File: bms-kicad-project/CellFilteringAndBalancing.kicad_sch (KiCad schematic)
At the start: 111 parts, among them J1 S13B-XH-A, Q1 DNBT8105-7, Q10 DNBT8105-7, Q11 DNBT8105-7, Q12 DNBT8105-7, Q2 DNBT8105-7, Q3 DNBT8105-7, Q4 DNBT8105-7, Q5 DNBT8105-7, Q6 DNBT8105-7, Q7 DNBT8105-7, Q8 DNBT8105-7, Q9 DNBT8105-7

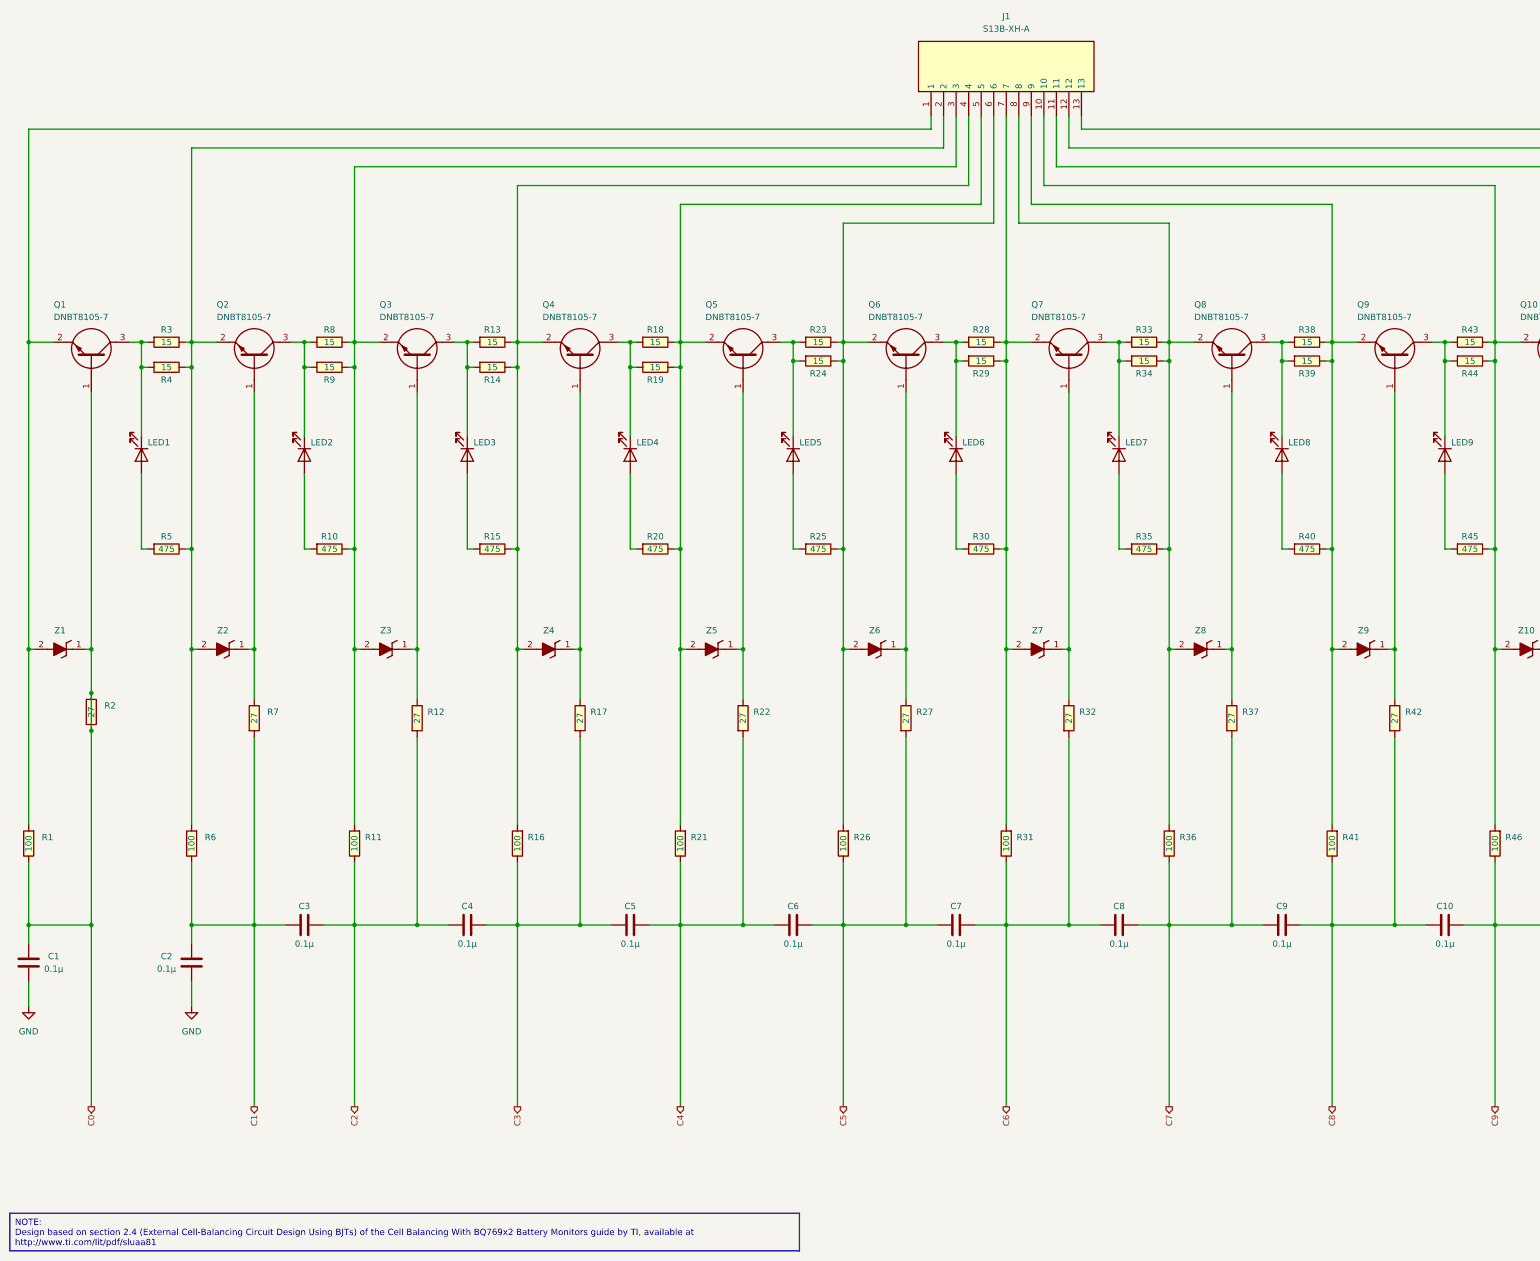
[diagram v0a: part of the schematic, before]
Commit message: feat: schematic pretty much done
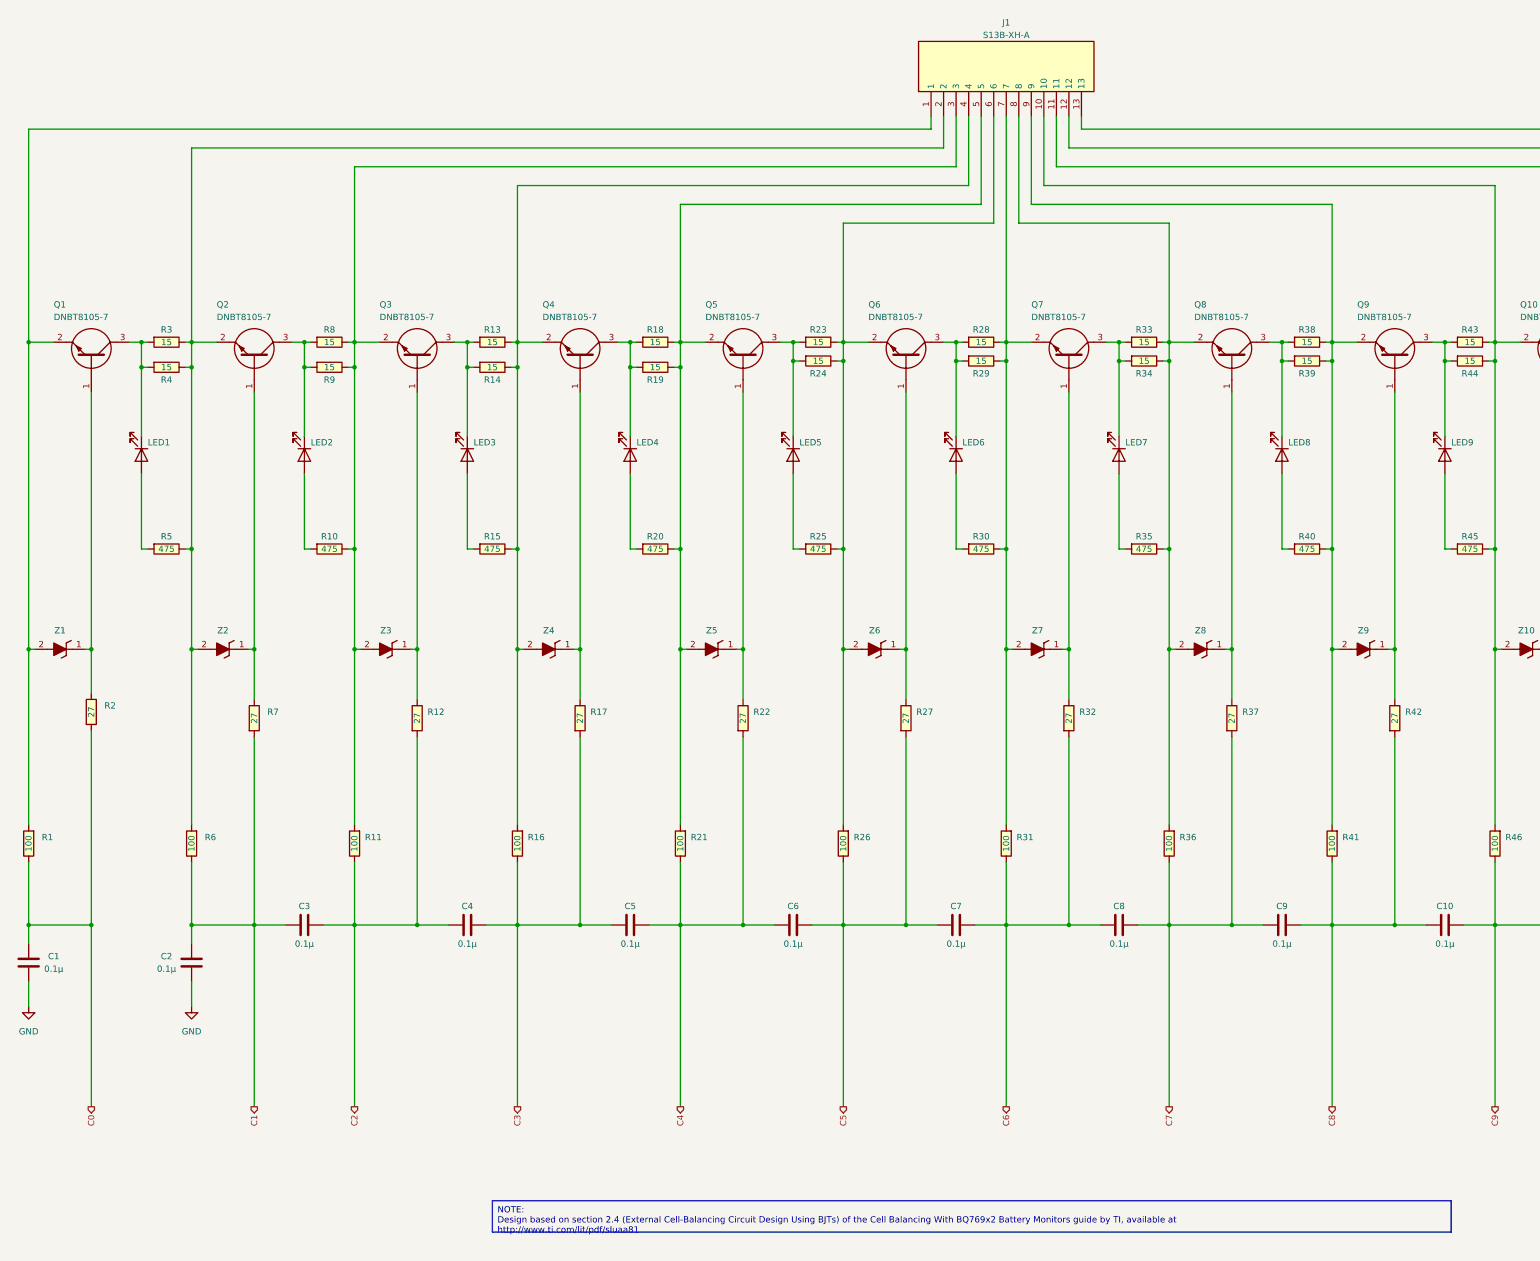
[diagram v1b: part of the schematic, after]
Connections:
- net C0: no longer Q1.1 (B), R2.2, Z1.1 (K)
- new net: Q1.1 (B), R2.2, Z1.1 (K)
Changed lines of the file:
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@@
   (title_block
     (title "Cell Filtering and Balancing")
-    (date "2024-08-10")
+    (date "2025-01-19")
     (rev "A")
     (company "AeroNU - FixedWing")
@@
   (junction (at 347.98 143.51) (diameter 0) (color 0 0 0 0)
   )
-  (junction (at 30.48 152.4) (diameter 0) (color 0 0 0 0)
-  )
   (junction (at 195.58 143.51) (diameter 0) (color 0 0 0 0)
   )
@@
   (junction (at 360.68 143.51) (diameter 0) (color 0 0 0 0)
   )
-  (junction (at 30.48 160.02) (diameter 0) (color 0 0 0 0)
-  )
   (junction (at 294.64 199.39) (diameter 0) (color 0 0 0 0)
   )
@@
     (stroke (width 0) (type default))
   )
-  (wire (pts (xy 30.48 152.4) (xy 30.48 160.02))
-    (stroke (width 0) (type default))
-  )
   (wire (pts (xy 379.73 85.09) (xy 381 85.09))
     (stroke (width 0) (type default))
@@
   )
   (text_box "NOTE:\nDesign based on section 2.4 (External Cell-Balancing Circuit Design Using BJTs) of the Cell Balancing With BQ769x2 Battery Monitors guide by TI, available at http://www.ti.com/lit/pdf/sluaa81"
-    (at 13.97 257.81 0) (size 160.02 7.62)
+    (at 111.76 255.27 0) (size 194.31 6.35)
     (stroke (width 0) (type default))
     (fill (type none))
-    (effects (font (size 1.27 1.27)) (justify left top))
+    (effects (font (size 1.27 1.27)) (justify left top) (href "http://www.ti.com/lit/pdf/sluaa81"))
   )
   (hierarchical_label "C10" (shape output) (at 347.98 236.22 270) (fields_autoplaced)
@@
   )
   (symbol (lib_id "FixedWing:S13B-XH-A") (at 200.66 35.56 90) (unit 1)
-    (in_bom yes) (on_board yes) (dnp no) (fields_autoplaced)
-    (property "Reference" "J1" (at 215.9 15.24 90)
-      (effects (font (size 1.27 1.27)))
-    )
-    (property "Value" "S13B-XH-A" (at 215.9 17.78 90)
+    (in_bom yes) (on_board yes) (dnp no)
+    (property "Reference" "J1" (at 215.9 16.51 90)
+      (effects (font (size 1.27 1.27)))
+    )
+    (property "Value" "S13B-XH-A" (at 215.9 19.05 90)
       (effects (font (size 1.27 1.27)))
     )
@@
   (symbol (lib_id "power:GND") (at 50.8 215.9 0) (unit 1)
     (in_bom yes) (on_board yes) (dnp no) (fields_autoplaced)
-    (property "Reference" "#PWR05" (at 50.8 222.25 0)
+    (property "Reference" "#PWR02" (at 50.8 222.25 0)
       (effects (font (size 1.27 1.27)) hide)
     )
@@
       (project "bms-board"
         (path "/8a7831d1-a913-4f04-8780-225d2234b41d/95f820cc-7b9f-45ce-aa8e-ca8cb50aec5e"
-          (reference "#PWR05") (unit 1)
+          (reference "#PWR02") (unit 1)
         )
       )
@@
   (symbol (lib_id "power:GND") (at 17.78 215.9 0) (unit 1)
     (in_bom yes) (on_board yes) (dnp no) (fields_autoplaced)
-    (property "Reference" "#PWR04" (at 17.78 222.25 0)
+    (property "Reference" "#PWR01" (at 17.78 222.25 0)
       (effects (font (size 1.27 1.27)) hide)
     )
@@
       (project "bms-board"
         (path "/8a7831d1-a913-4f04-8780-225d2234b41d/95f820cc-7b9f-45ce-aa8e-ca8cb50aec5e"
-          (reference "#PWR04") (unit 1)
-        )
-      )
+          (reference "#PWR01") (unit 1)
+        )
+      )
